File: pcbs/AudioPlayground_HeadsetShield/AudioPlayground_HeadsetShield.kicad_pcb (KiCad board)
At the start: 2 copper layers, 20.1 x 22.9 mm, 9 parts, among them J1 Conn_01x05_Socket, J3 SJ2-35364B-SMT-TR, J4 SJ2-35364B-SMT-TR, J9 Conn_01x05_Socket, SW1 SW_Push, SW2 SW_Push, SW3 SW_Push, SW4 SW_Push, SW5 SW_Push

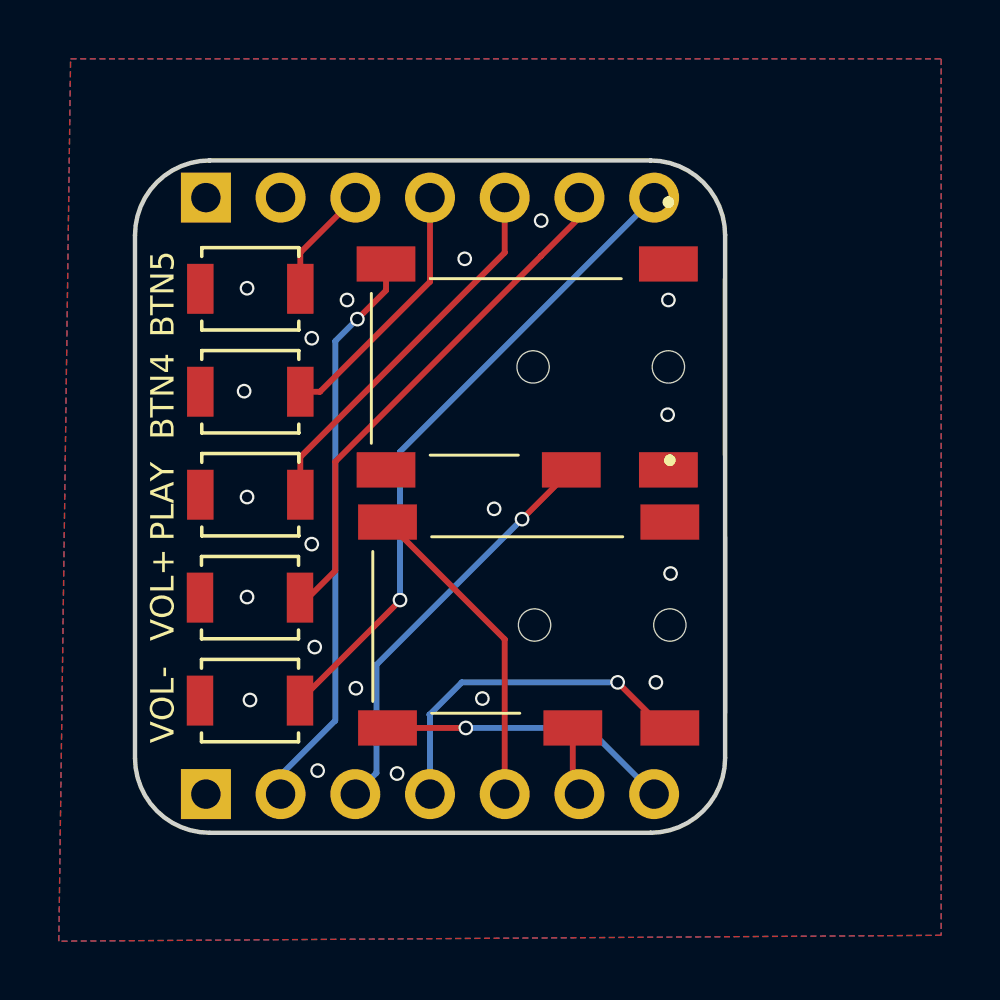
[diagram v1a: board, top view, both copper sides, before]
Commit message: Add HeadsetShield v2.0
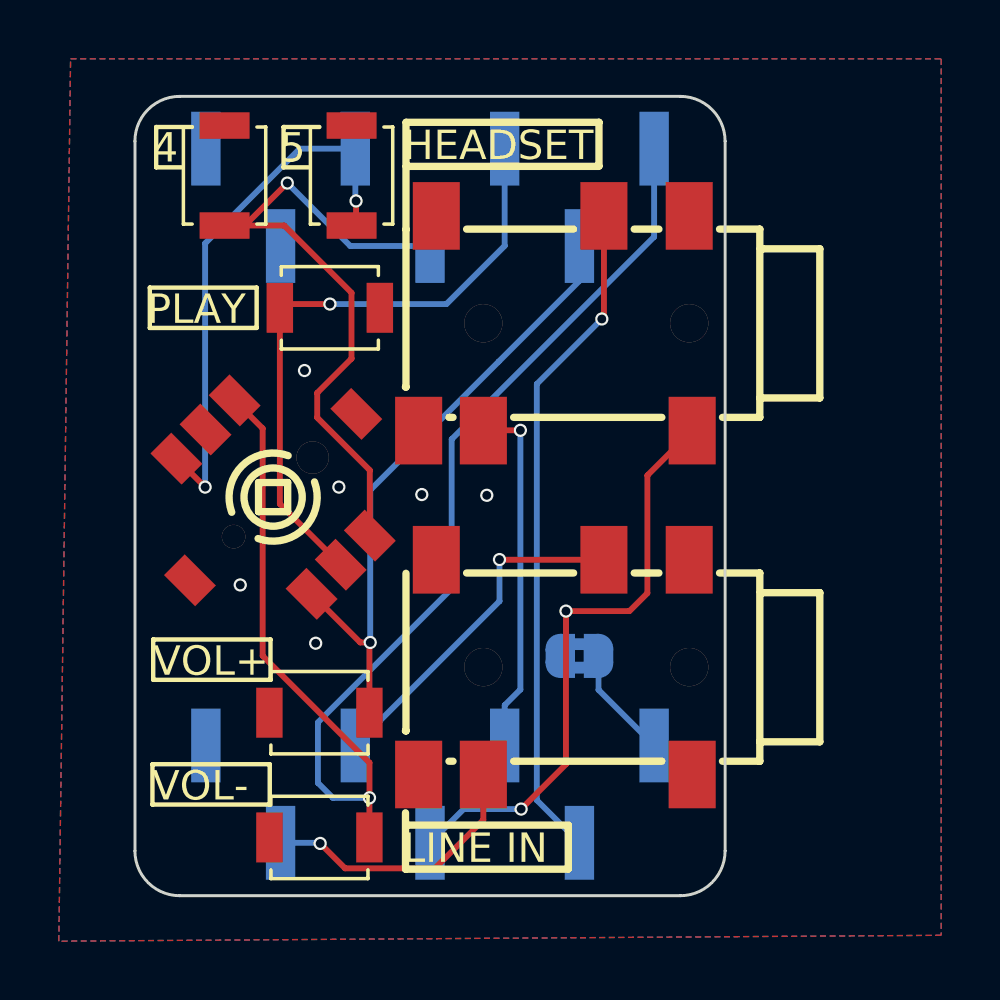
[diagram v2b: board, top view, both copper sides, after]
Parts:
- removed J1, J9: Conn_01x05_Socket, Connector_PinHeader_2.54mm:PinHeader_1x07_P2.54mm_Vertical
- removed J3, J4: SJ2-35364B-SMT-TR, SJ235364BSMTTR:SJ235364BSMTTR
- added CN1: PJ-342, PJ-342:PJ-342, F.Cu at (128.4, 99.7)
- added CN2: PJ-342, PJ-342:PJ-342, F.Cu at (128.4, 111.4)
- added G***: LOGO, LOGO, B.Cu at (126.1, 106.4)
- added J2: Conn_01x07_Socket, Connector_PinHeader_2.54mm:PinHeader_1x07_P2.54mm_Vertical_SMD_Pin1Left, B.Cu at (124.1, 95.4)
- added J5: Conn_01x07_Socket, Connector_PinHeader_2.54mm:PinHeader_1x07_P2.54mm_Vertical_SMD_Pin1Left, B.Cu at (124.1, 115.7)
- added JP1: Jumper_2_Bridged, Jumper:SolderJumper-2_P1.3mm_Bridged2Bar_RoundedPad1.0x1.5mm, B.Cu at (129.2, 111.0)
- added SW6: 7*7*5-6P-L WX, 7*7*5-6P-LWX:7*7*5-6P-LWX, F.Cu at (118.8, 105.6)
- moved SW4 7.40 mm to (117.1, 94.6), turned to 90 degrees
- moved SW3 6.91 mm to (120.7, 99.1), turned to 0 degrees
- moved SW1 5.22 mm to (120.4, 117.2)
- moved SW5 5.17 mm to (121.4, 94.6), turned to 90 degrees
- moved SW2 4.57 mm to (120.4, 112.9)
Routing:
- net /BTN1: track 22.1 -> 45.0 mm
- net /ROUTP: track 2.34 -> 22.9 mm, vias 0 -> 1
- net /BTN5: track 3.88 -> 18.7 mm, vias 0 -> 2
- net /BTN4: track 8.82 -> 23.2 mm, vias 0 -> 1
- net /LINL: track 19.5 -> 9.48 mm
- net /MIC: track 12.0 -> 21.7 mm, vias 1 -> 2
- net /BTN3: track 13.0 -> 21.3 mm, vias 0 -> 1
- net /JACKSNS: track 10.00 -> 3.83 mm, vias 1 -> 0
- net /BTN2: track 17.7 -> 21.5 mm, vias 0 -> 1
- net /LINR: track 14.1 -> 11.9 mm
- net /LOUTP: track 10.9 -> 12.2 mm, vias 0 -> 1
- net GND: vias 20 -> 6
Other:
- board size 20.1 x 22.9 mm -> 20.1 x 27.2 mm
- board text added: "4"
- board text added: "5"
- board text added: "HEADSET"
- board text added: "HeadsetShield v2.0"
- board text added: "LINE IN"
- board text removed: "BTN4"
- board text removed: "BTN5"

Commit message: Fix Naming
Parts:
- SW6: value 7*7*5-6P-L WX -> 775-6P-LWX
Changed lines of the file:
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@@
 			)
 		)
-		(property "Value" "7*7*5-6P-L WX"
+		(property "Value" "775-6P-LWX"
 			(at 0 8 135)
 			(layer "F.Fab")
@@
 		)
 		(embedded_fonts no)
-		(model "${KIPRJMOD}/../../components/7*7*5-6P-LWX/7*7*5-6P-LWX.step"
+		(model "${KIPRJMOD}/../../components/775-6P-LWX/775-6P-LWX.step"
 			(offset
 				(xyz 0 -0 1.8)
@@
 		(sheetfile "AudioPlayground_HeadsetShield.kicad_sch")
 		(zone_connect 1)
-		(attr exclude_from_pos_files exclude_from_bom allow_soldermask_bridges)
+		(attr exclude_from_pos_files allow_soldermask_bridges)
 		(net_tie_pad_groups "1, 2")
 		(fp_poly
